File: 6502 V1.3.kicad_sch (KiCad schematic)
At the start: 40 parts, among them J1 Conn_02x32_Odd_Even, J2 USB_C_Receptacle_USB2.0_16P, SW1 SW_Push, SW2 SW_DIP_x04, U1 ATF22V10B-15GM/883, U2 W65C02SxP, U3 W65C22SxP, U4 W65C51NxP, U5 SST39SF040, U6 FT230XS, U7 CY62256-70PC, X1 ACO-1.8432MHz-A, X2 ACO-1MHz-A

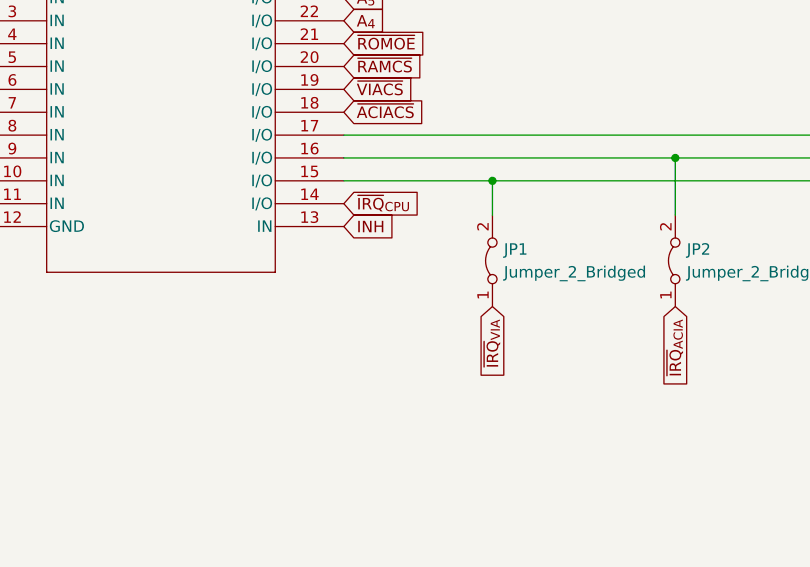
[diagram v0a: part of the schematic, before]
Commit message: Finished tracing, corrected INH pull resistor
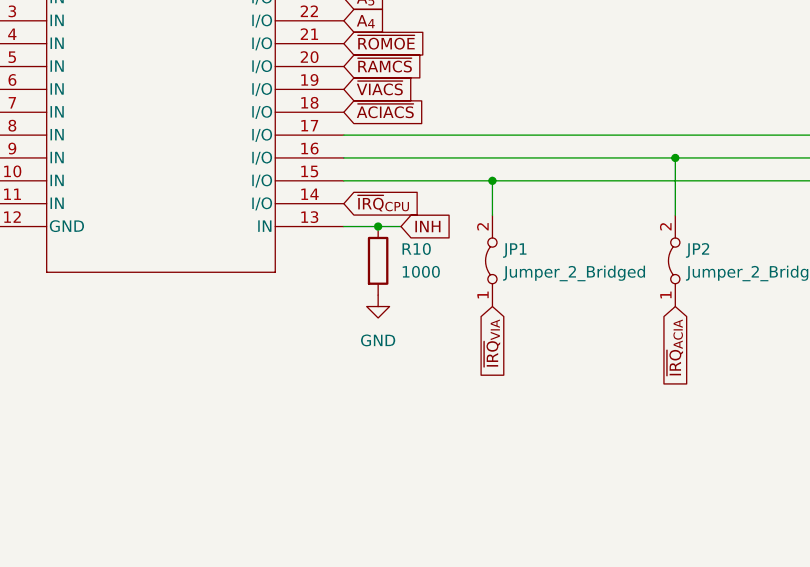
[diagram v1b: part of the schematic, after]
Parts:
- added R10: 1000, Resistor_SMD:R_1206_3216Metric, symbol Device:R
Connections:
- net GND: now also R10.2
- net INH: now also R10.1
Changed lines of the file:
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@@
   (junction (at 317.5 88.9) (diameter 0) (color 0 0 0 0)
   )
+  (junction (at 71.12 143.51) (diameter 0) (color 0 0 0 0)
+  )
   (junction (at 251.46 176.53) (diameter 0) (color 0 0 0 0)
   )
@@
     (stroke (width 0) (type default))
   )
+  (wire (pts (xy 71.12 143.51) (xy 73.66 143.51))
+    (stroke (width 0) (type default))
+  )
   (wire (pts (xy 251.46 176.53) (xy 259.08 176.53))
     (stroke (width 0) (type default))
@@
     (stroke (width 0) (type default))
   )
+  (wire (pts (xy 67.31 143.51) (xy 71.12 143.51))
+    (stroke (width 0) (type default))
+  )
   (wire (pts (xy 256.54 96.52) (xy 259.08 96.52))
     (stroke (width 0) (type default))
@@
     )
   )
-  (global_label "INH" (shape input) (at 67.31 143.51 0) (fields_autoplaced)
+  (global_label "INH" (shape input) (at 73.66 143.51 0) (fields_autoplaced)
     (effects (font (size 1.27 1.27)) (justify left))
-    (property "Intersheetrefs" "${INTERSHEET_REFS}" (at 73.561 143.51 0)
+    (property "Intersheetrefs" "${INTERSHEET_REFS}" (at 79.911 143.51 0)
       (effects (font (size 1.27 1.27)) (justify left) hide)
     )
@@
     )
   )
+  (symbol (lib_id "power:GND") (at 71.12 151.13 0) (unit 1)
+    (in_bom yes) (on_board yes) (dnp no) (fields_autoplaced)
+    (property "Reference" "#PWR066" (at 71.12 157.48 0)
+      (effects (font (size 1.27 1.27)) hide)
+    )
+    (property "Value" "GND" (at 71.12 156.21 0)
+      (effects (font (size 1.27 1.27)))
+    )
+    (property "Footprint" "" (at 71.12 151.13 0)
+      (effects (font (size 1.27 1.27)) hide)
+    )
+    (property "Datasheet" "" (at 71.12 151.13 0)
+      (effects (font (size 1.27 1.27)) hide)
+    )
+    (pin "1")
+    (instances
+      (project "6502 V1.3"
+        (path "/2462ee6a-a1ab-4fa8-8d76-c1bc8dad46c9"
+          (reference "#PWR066") (unit 1)
+        )
+      )
+    )
+  )
   (symbol (lib_id "power:VCC") (at 220.98 83.82 90) (unit 1)
     (in_bom yes) (on_board yes) (dnp no) (fields_autoplaced)
@@
         )
       )
+    )
+  )
+  (symbol (lib_id "Device:R") (at 71.12 147.32 0) (unit 1)
+    (in_bom yes) (on_board yes) (dnp no) (fields_autoplaced)
+    (property "Reference" "R10" (at 73.66 146.05 0)
+      (effects (font (size 1.27 1.27)) (justify left))
+    )
+    (property "Value" "1000" (at 73.66 148.59 0)
+      (effects (font (size 1.27 1.27)) (justify left))
+    )
+    (property "Footprint" "Resistor_SMD:R_1206_3216Metric" (at 69.342 147.32 90)
+      (effects (font (size 1.27 1.27)) hide)
+    )
+    (property "Datasheet" "~" (at 71.12 147.32 0)
+      (effects (font (size 1.27 1.27)) hide)
+    )
+    (pin "1")
+    (pin "2")
+    (instances
+      (project "6502 V1.3"
+        (path "/2462ee6a-a1ab-4fa8-8d76-c1bc8dad46c9"
+          (reference "R10") (unit 1)
+        )
+      )
